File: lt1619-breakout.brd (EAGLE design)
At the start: 39.4 x 24.1 mm, 20 parts

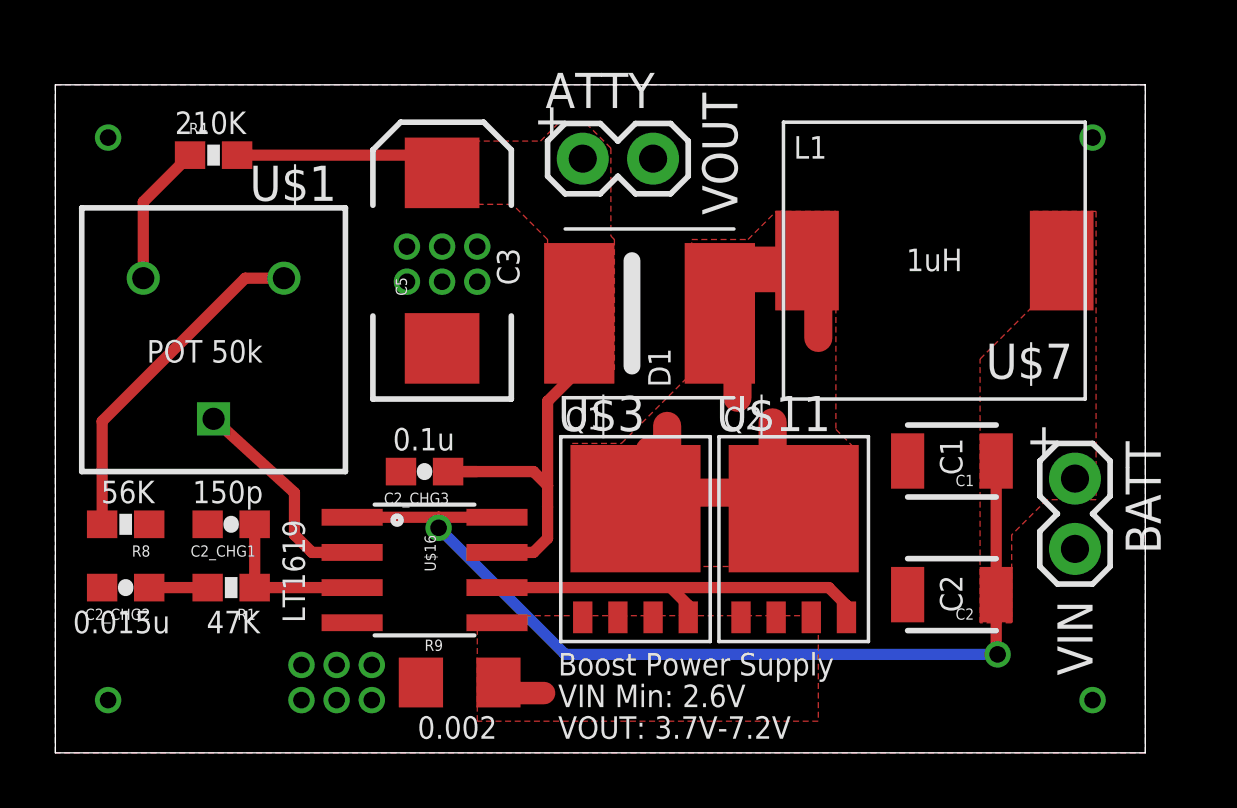
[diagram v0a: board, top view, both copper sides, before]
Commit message: schematic cleanup
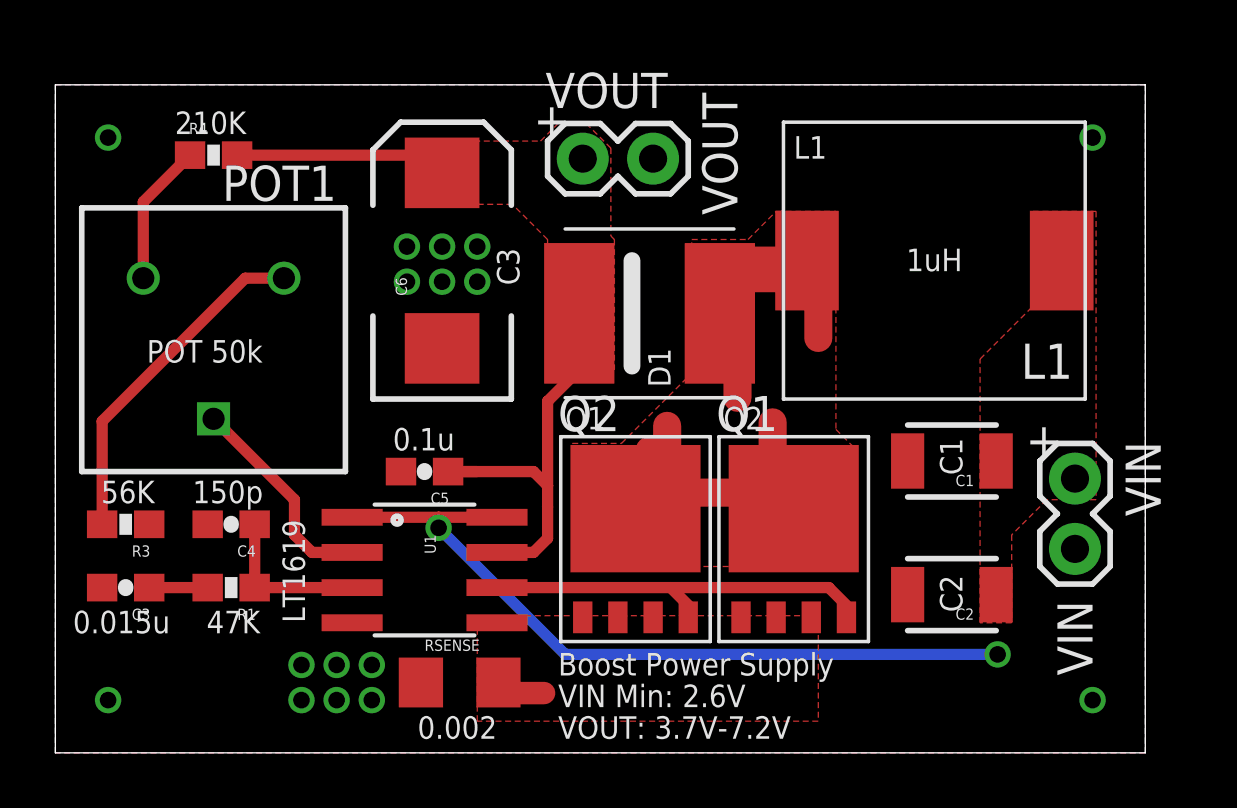
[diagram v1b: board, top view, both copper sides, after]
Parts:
- removed C2_CHG3: 0.1u, SparkFun:0603-CAP
- added C6: 220u, SparkFun-Passives:EIA7343
- C5: value 220u -> 0.1u; device SparkFun-Passives:EIA7343 -> SparkFun:0603-CAP
- D1: value SCHOTTKYDO214AB -> 20V
- POT1: value POT3310Y-001 -> 50K
- Q1, Q2: value MOSFET_NP-S08 -> P-CHAN
- moved C5 7.65 mm to (13.3, 10.2), turned to 180 degrees
- renumbered ATTY to VOUT, BATT to VIN, C2_CHG1 to C4, C2_CHG2 to C3, R8 to R3, R9 to RSENSE, U$1 to POT1, U$10 to D1, U$11 to Q1, U$16 to U1, U$3 to Q2, U$7 to L1
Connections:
- net N$16 renamed FB
- net N$3 renamed DRAIN
- net N$4 renamed GATE
- net N$7 renamed SOURCE
- net V_BATT renamed VBATT
- removed net V_ATTY: C2_CHG3.1, C5.A, D1.C, R4.2, U1.7, VOUT.1
- new net VOUT: C5.1, C6.A, D1.C, R4.2, U1.7, VOUT.1
- net GND: now also C5.2, C6.C; no longer C2_CHG3.2, C5.C
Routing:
- net V_ATTY: track 23.2 -> 0.00 mm
- net VOUT: track 0.00 -> 21.3 mm
- net VBATT: track 34.7 -> 27.8 mm
- net GATE: track 14.7 -> 13.8 mm
- added copper zone on layer 1, net VOUT
- removed copper zone on layer 1, net V_ATTY
